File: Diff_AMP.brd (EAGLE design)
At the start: 34.4 x 13.5 mm, 24 parts, among them IC1 NCV8711ASN500T1G, IC3 MCP1501T-25E_RW, IC4 NCS21911SN2T1G, IC5 NCS21911SN2T1G

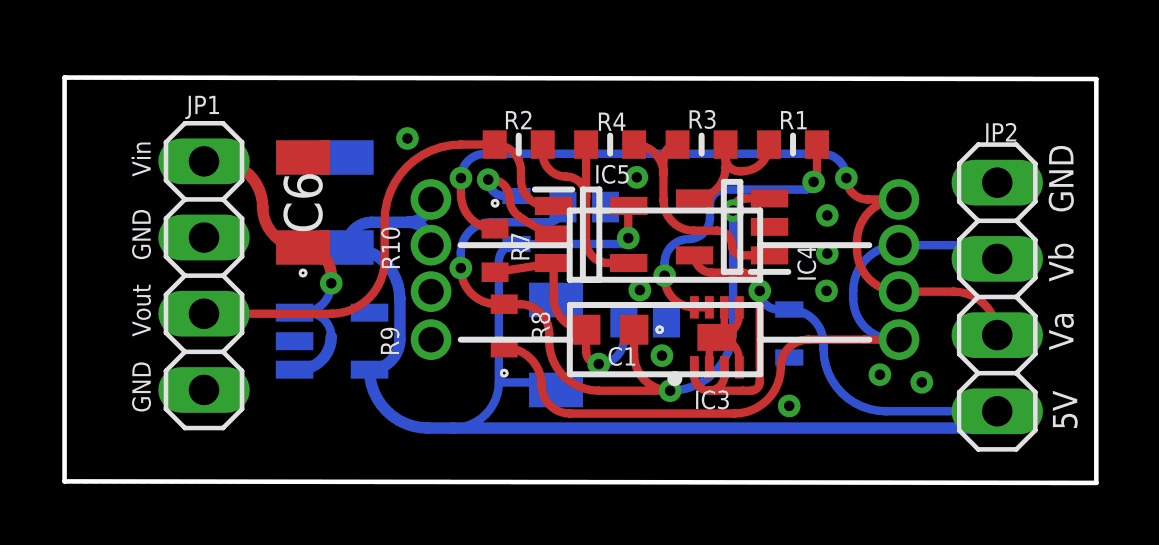
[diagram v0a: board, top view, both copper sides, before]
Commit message: revision
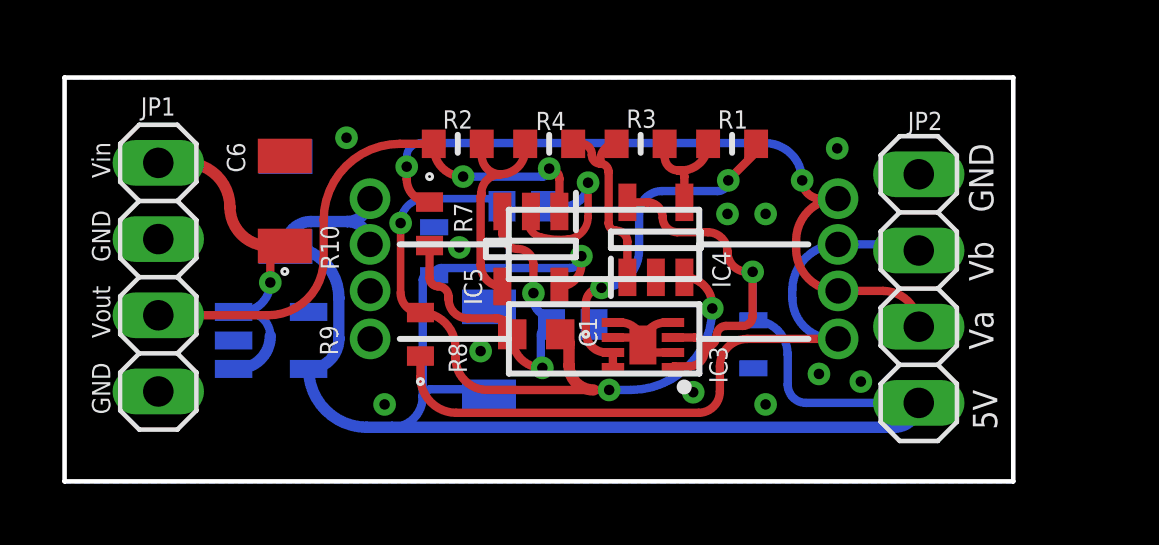
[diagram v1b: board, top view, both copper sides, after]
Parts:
- moved C5 2.93 mm to (12.3, 7.67)
- moved R8 2.81 mm to (11.8, 4.90)
- moved JP2 2.63 mm to (28.5, 6.43)
- moved IC4 2.58 mm to (19.7, 8.05), turned to 90 degrees
- moved IC3 2.48 mm to (19.3, 4.55), turned to 180 degrees
- moved C1 2.47 mm to (15.7, 4.90)
- moved C2 2.41 mm to (16.9, 5.23)
- moved R7 2.36 mm to (12.2, 8.59)
- moved C3 2.25 mm to (14.1, 4.32)
- moved IC5 2.06 mm to (15.5, 7.75), turned to 270 degrees
- moved C7 2.03 mm to (7.37, 9.32)
- moved C8 2.03 mm to (15.3, 9.17)
- moved IC1 2.03 mm to (6.88, 4.70)
- moved R1 2.03 mm to (22.3, 11.3)
- moved R10 2.03 mm to (25.8, 7.90)
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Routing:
- net N$9: track 7.71 -> 12.3 mm, vias 1 -> 2
- net VOUT: track 15.8 -> 18.4 mm, vias 0 -> 2
- net GND: track 8.95 -> 10.6 mm, vias 11 -> 12
- net N$12: track 7.73 -> 6.24 mm
- net N$1: track 10.0 -> 11.4 mm
- net 5V: track 64.8 -> 66.2 mm
- net VA: track 25.8 -> 24.6 mm
- net N$3: track 24.2 -> 22.9 mm
- net VB: track 23.1 -> 23.9 mm
- net VIN: track 10.9 -> 11.6 mm
- net N$2: track 4.23 -> 3.58 mm
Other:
- board size 34.4 x 13.5 mm -> 31.6 x 13.5 mm

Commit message: Sent to Fab
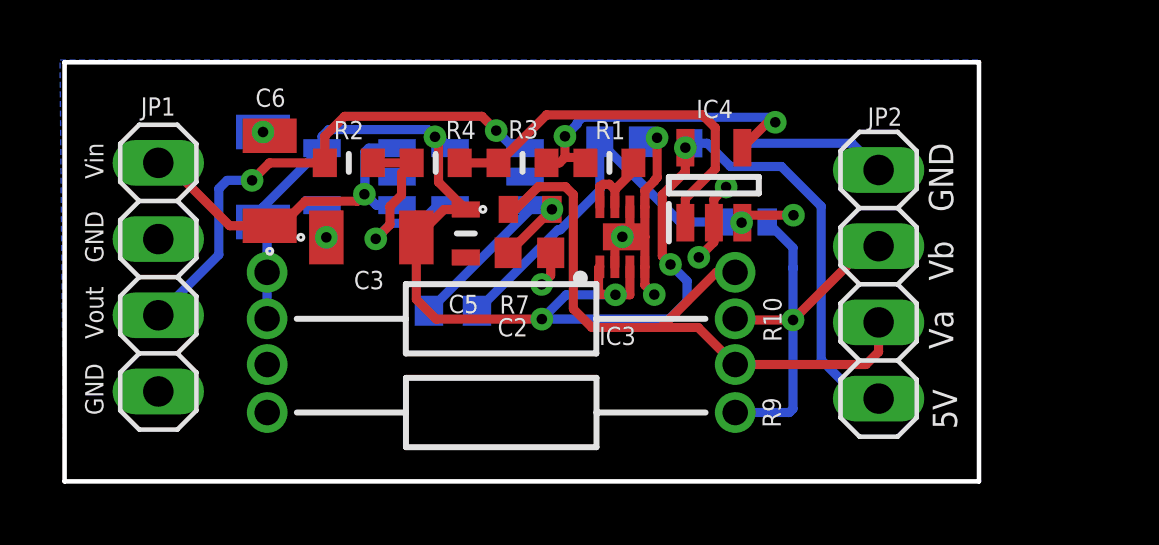
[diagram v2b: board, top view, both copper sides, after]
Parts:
- moved R8 11.5 mm to (22.7, 8.67), flipped to the bottom, turned to 0 degrees
- moved C4 6.80 mm to (21.8, 11.3), turned to 0 degrees
- moved IC1 6.21 mm to (9.83, 10.2), turned to 0 degrees
- moved C3 5.47 mm to (10.2, 8.14), flipped to the top, turned to 0 degrees
- moved R10 4.23 mm to (22.4, 5.42)
- moved R5 4.22 mm to (22.4, 6.97)
- moved R6 4.22 mm to (6.75, 3.90)
- moved R9 4.22 mm to (6.75, 2.30)
- moved R1 4.14 mm to (18.2, 10.6)
- moved R3 3.99 mm to (15.3, 10.6)
- moved C8 3.91 mm to (18.6, 11.3)
- moved R4 3.84 mm to (12.4, 10.6)
- moved R2 3.69 mm to (9.47, 10.6)
- moved IC3 3.67 mm to (18.6, 8.15), turned to 90 degrees
- moved R7 3.37 mm to (15.5, 9.09), turned to 0 degrees
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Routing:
- net 5V: track 66.2 -> 52.5 mm, vias 2 -> 5
- net VB: track 23.9 -> 14.4 mm, vias 0 -> 1
- net N$1: track 11.4 -> 3.01 mm, vias 2 -> 0
- net GND: track 10.6 -> 18.1 mm, vias 12 -> 8
- net N$2: track 3.58 -> 11.0 mm, vias 0 -> 2
- net N$3: track 22.9 -> 15.7 mm, vias 3 -> 2
- net N$12: track 6.24 -> 12.9 mm
- net N$9: track 12.3 -> 8.51 mm, vias 2 -> 1
- net VA: track 24.6 -> 21.7 mm, vias 2 -> 0
- net VOUT: track 18.4 -> 17.2 mm
- net N$13: track 6.95 -> 7.27 mm, vias 0 -> 1
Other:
- board size 31.6 x 13.5 mm -> 30.5 x 14 mm
